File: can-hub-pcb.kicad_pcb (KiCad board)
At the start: 2 copper layers, 42.1 x 33.6 mm, 11 parts, among them J1 CAN_1, J2 CAN_2, J3 CAN_3, J4 CAN_TERM

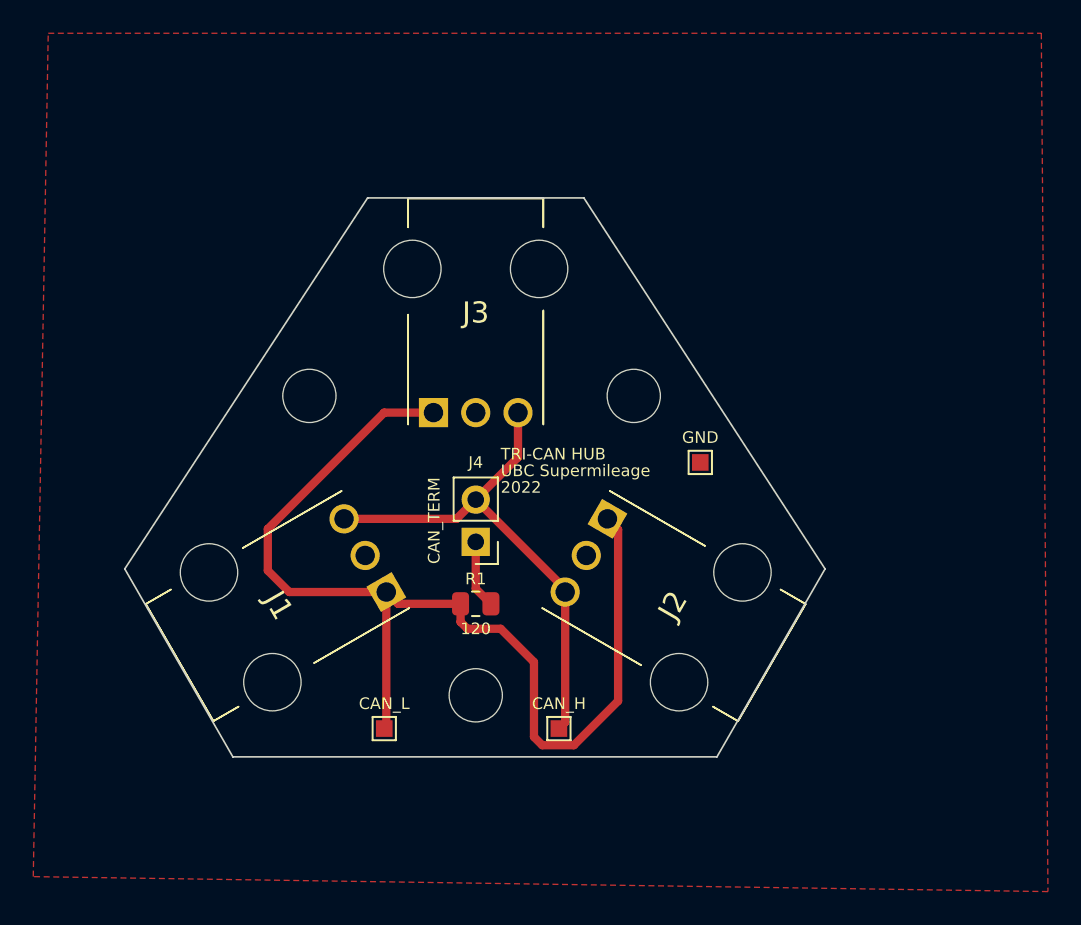
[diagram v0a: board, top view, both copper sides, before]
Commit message: finishes PCB and exports output
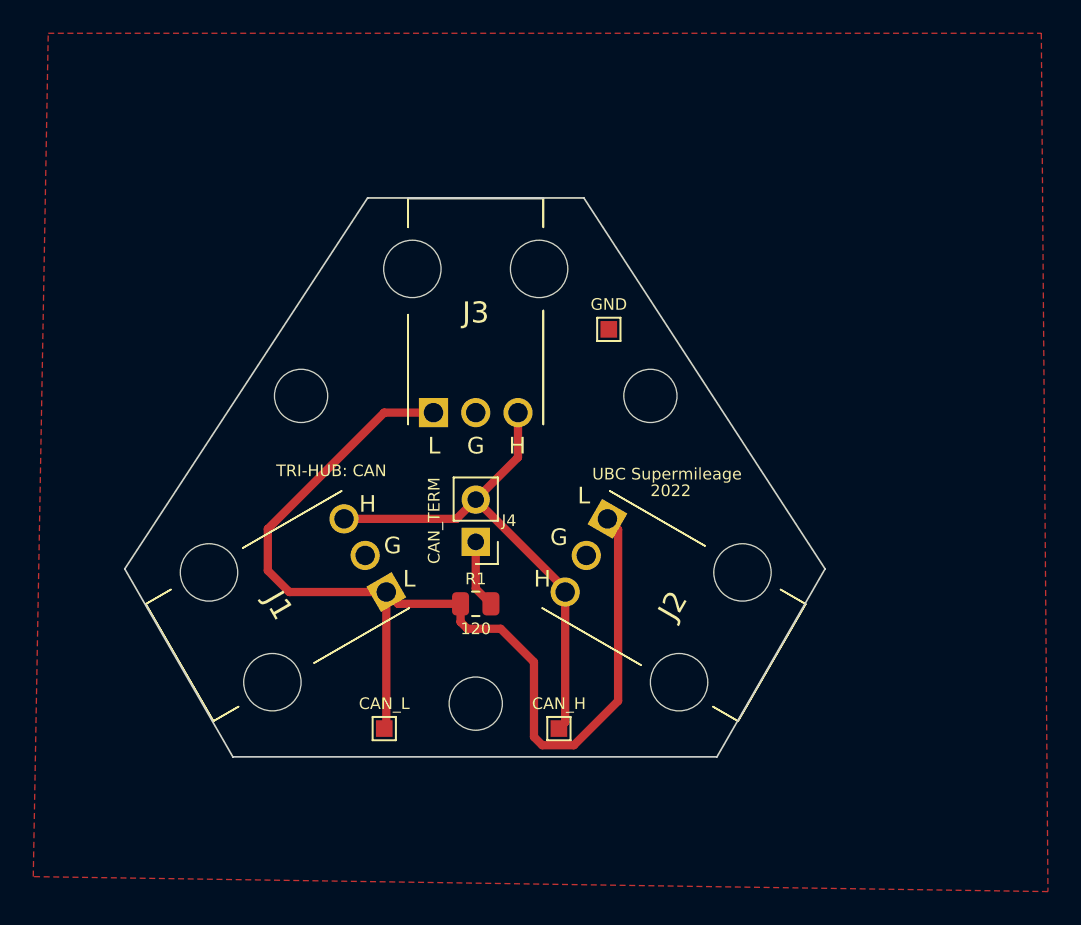
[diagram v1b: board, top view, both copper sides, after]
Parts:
- moved TP2 9.71 mm to (165.5, 88.0)
- moved H1 1.00 mm to (168.0, 92.0)
- moved H2 0.50 mm to (157.5, 110.5)
- moved H3 0.50 mm to (147.0, 92.0)
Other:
- board text added: "G"
- board text added: "H"
- board text added: "L"
- board text added: "TRI-HUB: CAN"
- board text removed: "TRI-CAN HUB"
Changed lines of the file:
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@@
       (layerselection 0x00010fc_ffffffff)
       (disableapertmacros false)
-      (usegerberextensions false)
-      (usegerberattributes true)
-      (usegerberadvancedattributes true)
-      (creategerberjobfile true)
+      (usegerberextensions true)
+      (usegerberattributes false)
+      (usegerberadvancedattributes false)
+      (creategerberjobfile false)
       (svguseinch false)
       (svgprecision 6)
@@
       (plotinvisibletext false)
       (sketchpadsonfab false)
-      (subtractmaskfromsilk false)
+      (subtractmaskfromsilk true)
       (outputformat 1)
       (mirror false)
-      (drillshape 1)
+      (drillshape 0)
       (scaleselection 1)
-      (outputdirectory "")
+      (outputdirectory "output")
     )
   )
@@
     (property "Sheetname" "")
     (attr through_hole)
-    (fp_text reference "J4" (at 0 4.775) (layer "F.SilkS")
+    (fp_text reference "J4" (at -2 1.275) (layer "F.SilkS")
       (effects (font (size 0.7 0.7) (thickness 0.15)))
     )
@@
     (fp_line (start 1 -0.625) (end 1 0.625) (layer "F.Fab") (width 0.1))
     (fp_line (start 1 0.625) (end -1 0.625) (layer "F.Fab") (width 0.1))
-    (pad "1" smd roundrect (at -0.9125 0 180) (size 1.025 1.4) (layers "F.Cu" "F.Paste" "F.Mask") (roundrect_rratio 0.243902)
+    (pad "1" smd roundrect (at -0.9125 0 180) (size 1.025 1.4) (layers "F.Cu" "F.Paste" "F.Mask") (roundrect_rratio 0.243902439)
       (net 4 "Net-(J4-Pad1)") (pintype "passive"))
-    (pad "2" smd roundrect (at 0.9125 0 180) (size 1.025 1.4) (layers "F.Cu" "F.Paste" "F.Mask") (roundrect_rratio 0.243902)
+    (pad "2" smd roundrect (at 0.9125 0 180) (size 1.025 1.4) (layers "F.Cu" "F.Paste" "F.Mask") (roundrect_rratio 0.243902439)
       (net 2 "CAN_L") (pintype "passive"))
     (model "${KICAD6_3DMODEL_DIR}/Resistor_SMD.3dshapes/R_0805_2012Metric.wrl"
@@
   )
   (footprint "MountingHole:MountingHole_3.2mm_M3" (layer "F.Cu")
-    (at 157.5 110)
+    (at 157.5 110.5)
     (descr "Mounting Hole 3.2mm, no annular, M3")
     (tags "mounting hole 3.2mm no annular m3")
@@
   )
   (footprint "TestPoint:TestPoint_Pad_1.0x1.0mm" (layer "F.Cu")
-    (at 171 96)
+    (at 165.5 88)
     (descr "SMD rectangular pad as test Point, square 1.0mm side length")
     (tags "test point SMD pad rectangle square")
@@
   )
   (footprint "MountingHole:MountingHole_3.2mm_M3" (layer "F.Cu")
-    (at 167 92)
+    (at 168 92)
     (descr "Mounting Hole 3.2mm, no annular, M3")
     (tags "mounting hole 3.2mm no annular m3")
@@
   )
   (footprint "MountingHole:MountingHole_3.2mm_M3" (layer "F.Cu")
-    (at 147.5 92)
+    (at 147 92)
     (descr "Mounting Hole 3.2mm, no annular, M3")
     (tags "mounting hole 3.2mm no annular m3")
@@
   (gr_line (start 178.5 102.4) (end 164 80.1) (layer "Edge.Cuts") (width 0.1))
   (gr_line (start 172 113.7) (end 178.5 102.4) (layer "Edge.Cuts") (width 0.1))
-  (gr_text "UBC Supermileage\n" (at 159 96.5) (layer "F.SilkS")
+  (gr_text "UBC Supermileage\n" (at 164.5 96.7) (layer "F.SilkS")
     (effects (font (size 0.7 0.7) (thickness 0.15)) (justify left))
   )
-  (gr_text "2022" (at 159 97.5) (layer "F.SilkS")
+  (gr_text "G" (at 152.5 101) (layer "F.SilkS")
+    (effects (font (size 1 1) (thickness 0.15)))
+  )
+  (gr_text "L" (at 153.5 103) (layer "F.SilkS")
+    (effects (font (size 1 1) (thickness 0.15)))
+  )
+  (gr_text "G" (at 162.5 100.5) (layer "F.SilkS")
+    (effects (font (size 1 1) (thickness 0.15)))
+  )
+  (gr_text "L" (at 155 95) (layer "F.SilkS")
+    (effects (font (size 1 1) (thickness 0.15)))
+  )
+  (gr_text "H" (at 161.5 103) (layer "F.SilkS")
+    (effects (font (size 1 1) (thickness 0.15)))
+  )
+  (gr_text "2022" (at 168 97.7) (layer "F.SilkS")
     (effects (font (size 0.7 0.7) (thickness 0.15)) (justify left))
   )
-  (gr_text "TRI-CAN HUB" (at 159 95.5) (layer "F.SilkS")
+  (gr_text "G" (at 157.5 95) (layer "F.SilkS")
+    (effects (font (size 1 1) (thickness 0.15)))
+  )
+  (gr_text "H" (at 151 98.5) (layer "F.SilkS")
+    (effects (font (size 1 1) (thickness 0.15)))
+  )
+  (gr_text "L" (at 164 98) (layer "F.SilkS")
+    (effects (font (size 1 1) (thickness 0.15)))
+  )
+  (gr_text "H" (at 160 95) (layer "F.SilkS")
+    (effects (font (size 1 1) (thickness 0.15)))
+  )
+  (gr_text "TRI-HUB: CAN" (at 145.5 96.5) (layer "F.SilkS")
     (effects (font (size 0.7 0.7) (thickness 0.15)) (justify left))
   )
